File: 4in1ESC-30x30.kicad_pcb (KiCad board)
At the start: 6 copper layers, 41.6 x 42.5 mm, 226 parts, among them J1 SM08B-SRSS-TB, Q1 C22385416, Q10 C22385416, Q11 C22385416, Q12 C22385416, Q13 C22385416, Q14 C22385416, Q15 C22385416, Q16 C22385416, Q17 C22385416, Q18 C22385416, Q19 C22385416, Q2 C22385416, Q20 C22385416, Q21 C22385416, Q22 C22385416, Q23 C22385416, Q24 C22385416, Q3 C22385416, Q4 C22385416, Q5 C22385416, Q6 C22385416, Q7 C22385416, Q8 C22385416, Q9 C22385416, U1 TLV76733DRVR, U10 AT32F421G8U7, U11 NSG2065Q, U12 INA186A3IDCKR, U18 LMR51420YDDCR, U2 AT32F421G8U7, U4 NSG2065Q, U5 XRIM160808SR47MBCD, U6 AT32F421G8U7, U7 NSG2065Q, U8 AT32F421G8U7, U9 NSG2065Q

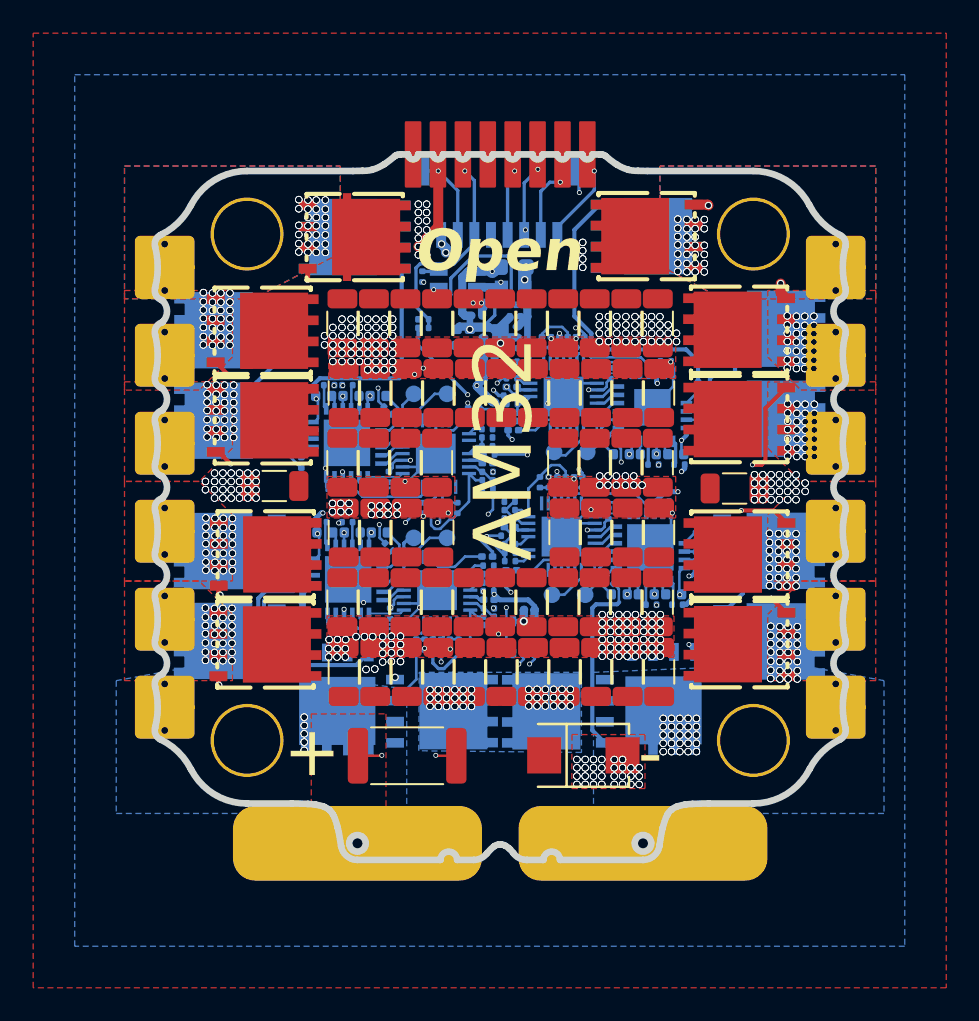
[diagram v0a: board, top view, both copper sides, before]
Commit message: alpha routing
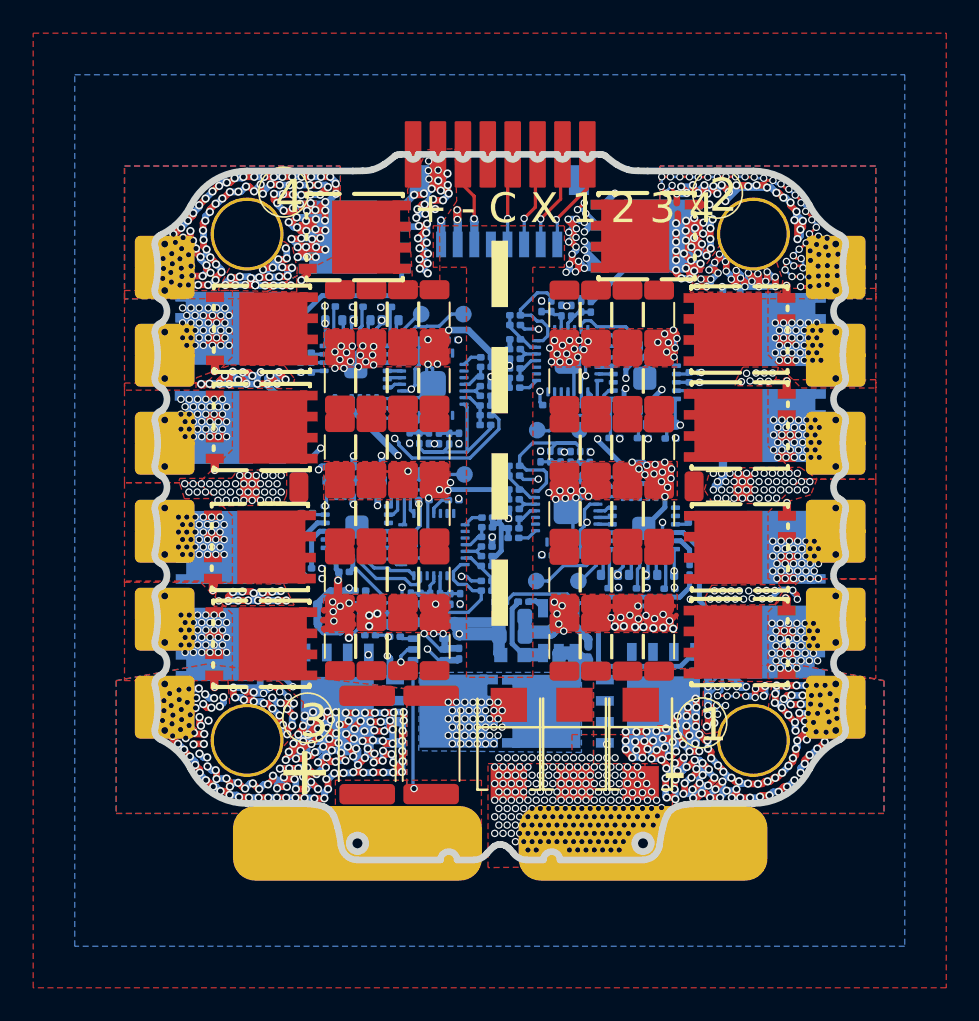
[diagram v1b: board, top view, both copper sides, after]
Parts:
- removed C1, C42: 22uF, Capacitor_SMD:C_0402_1005Metric
- removed C46, C77, C78: 100nF, Capacitor_SMD:C_0201_0603Metric
- removed the C6 at (81.3, 37.5)
- removed the C6 at (83.2, 45.9)
- removed the C6 at (83.2, 37.5)
- removed the C6 at (66.2, 50.1)
- removed the C6 at (70.0, 41.7)
- removed the C6 at (66.2, 41.7)
- removed the C6 at (68.0, 54.3)
- removed the C6 at (73.7, 37.5)
- removed the C6 at (77.6, 58.5)
- removed the C6 at (75.7, 58.5)
- removed the C6 at (68.1, 50.1)
- removed the C6 at (79.5, 41.7)
- removed the C6 at (71.8, 54.3)
- removed the C6 at (85.2, 58.5)
- removed the C6 at (71.8, 37.5)
- removed the C6 at (69.9, 37.5)
- removed the C6 at (71.8, 45.9)
- removed the C6 at (75.7, 41.7)
- removed the C6 at (73.7, 54.3)
- removed the C6 at (77.5, 54.3)
- removed the C6 at (79.5, 58.5)
- removed the C6 at (69.9, 45.9)
- removed the C6 at (81.3, 45.9)
- removed the C6 at (81.3, 54.3)
- removed the C6 at (73.8, 41.7)
- removed the C6 at (83.3, 50.1)
- removed the C6 at (75.6, 54.3)
- removed the C6 at (81.4, 41.7)
- removed the C6 at (75.6, 37.5)
- removed the C6 at (85.1, 54.3)
- removed the C6 at (79.5, 50.1)
- removed the C6 at (71.9, 58.5)
- removed the C6 at (73.8, 58.5)
- removed the C6 at (77.5, 37.5)
- removed the C6 at (79.4, 54.3)
- removed the C6 at (85.1, 37.5)
- removed the C6 at (85.2, 41.7)
- removed the C6 at (85.1, 45.9)
- removed the C6 at (71.9, 50.1)
- removed the C6 at (66.1, 54.3)
- removed the C6 at (83.3, 41.7)
- removed the C6 at (85.2, 50.1)
- removed the C6 at (79.4, 45.9)
- removed the C6 at (81.4, 50.1)
- removed the C6 at (68.1, 41.7)
- removed the C6 at (66.1, 45.9)
- removed the C6 at (68.0, 45.9)
- removed the C6 at (66.1, 37.5)
- removed the C6 at (83.3, 58.5)
- removed the C6 at (70.0, 58.5)
- removed the C6 at (71.9, 41.7)
- removed the C6 at (81.4, 58.5)
- removed the C6 at (79.4, 37.5)
- removed the C6 at (66.2, 58.5)
- removed the C6 at (69.9, 54.3)
- removed the C6 at (68.1, 58.5)
- removed the C6 at (70.0, 50.1)
- removed the C6 at (68.0, 37.5)
- removed the C6 at (77.6, 41.7)
- removed the C6 at (83.2, 54.3)
- removed C73: 100nF, Capacitor_SMD:C_0402_1005Metric
- removed FB1, FB2, FB3, FB4: BLM03PX121SN1D, Inductor_SMD:L_0201_0603Metric
- removed R1, R16, R17, R2, R6, R7, R8, R9: 8R, Capacitor_SMD:C_0201_0603Metric
- removed R118, R3, R4: 10k, Capacitor_SMD:C_0201_0603Metric
- removed R119: 124k, Resistor_SMD:R_0201_0603Metric
- removed R5: 220R, Resistor_SMD:R_0201_0603Metric
- removed U1: TLV76733DRVR, 4in1ESC-30x30:WSON-6_L2.0-W2.0-P0.65-TL-EP
- removed U11: NSG2065Q, 4in1ESC-30x30:QFN-24_L4.0-W4.0-P0.50-TL-EP2.8
- removed U18: LMR51420YDDCR, 4in1ESC-30x30:SOT-23-6_L2.9-W1.6-P0.95-LS2.9-BL
- added C100: 10uF, Capacitor_SMD:C_1206_3216Metric, F.Cu at (69.8, 56.9)
- added C101: 10uF, Capacitor_SMD:C_1206_3216Metric, F.Cu at (71.7, 56.9)
- added C105: 10uF, Capacitor_SMD:C_1206_3216Metric, F.Cu at (79.5, 57.0)
- added C106: 10uF, Capacitor_SMD:C_1206_3216Metric, F.Cu at (81.4, 57.0)
- added C107: 10uF, Capacitor_SMD:C_1206_3216Metric, F.Cu at (83.3, 57.0)
- added C108: 10uF, Capacitor_SMD:C_1206_3216Metric, F.Cu at (85.2, 57.0)
- added C13: 10uF, Capacitor_SMD:C_1206_3216Metric, F.Cu at (85.2, 37.0)
- added C14: 10uF, Capacitor_SMD:C_1206_3216Metric, F.Cu at (83.3, 37.0)
- added C15: 10uF, Capacitor_SMD:C_1206_3216Metric, F.Cu at (81.4, 37.0)
- added C16: 10uF, Capacitor_SMD:C_1206_3216Metric, F.Cu at (79.5, 37.0)
- added C17: 10uF, Capacitor_SMD:C_1206_3216Metric, F.Cu at (66.0, 40.9)
- added C18: 10uF, Capacitor_SMD:C_1206_3216Metric, F.Cu at (67.9, 40.9)
- added C19: 10uF, Capacitor_SMD:C_1206_3216Metric, F.Cu at (69.8, 40.9)
- added C20: 10uF, Capacitor_SMD:C_1206_3216Metric, F.Cu at (71.7, 40.9)
- added C24: 10uF, Capacitor_SMD:C_1206_3216Metric, F.Cu at (79.5, 41.0)
- added C25: 10uF, Capacitor_SMD:C_1206_3216Metric, F.Cu at (81.4, 41.0)
- added C26: 10uF, Capacitor_SMD:C_1206_3216Metric, F.Cu at (83.3, 41.0)
- added C27: 10uF, Capacitor_SMD:C_1206_3216Metric, F.Cu at (85.2, 41.0)
- added C28: 10uF, Capacitor_SMD:C_1206_3216Metric, F.Cu at (71.7, 44.9)
- added C29: 10uF, Capacitor_SMD:C_1206_3216Metric, F.Cu at (69.8, 44.9)
- added C30: 10uF, Capacitor_SMD:C_1206_3216Metric, F.Cu at (67.9, 44.9)
- added C31: 10uF, Capacitor_SMD:C_1206_3216Metric, F.Cu at (66.0, 44.9)
- added C4: 22uF, Capacitor_SMD:C_0402_1005Metric, B.Cu at (65.1, 54.5)
- added C47: 22uF, Capacitor_SMD:C_0603_1608Metric, B.Cu at (76.3, 55.1)
- added C51: 22uF, Capacitor_SMD:C_0402_1005Metric, B.Cu at (65.1, 55.4)
- added C52: 100nF, Capacitor_SMD:C_0201_0603Metric, B.Cu at (76.5, 40.8)
- added C54: 100nF, Capacitor_SMD:C_0201_0603Metric, B.Cu at (76.5, 39.0)
- added C55: 100nF, Capacitor_SMD:C_0201_0603Metric, B.Cu at (80.3, 42.4)
- added C56: 100nF, Capacitor_SMD:C_0402_WIDE, B.Cu at (82.3, 43.6)
- added C58: 100nF, Capacitor_SMD:C_0201_0603Metric, B.Cu at (85.1, 38.1)
- added C6: 10uF, Capacitor_SMD:C_1206_3216Metric, F.Cu at (79.5, 45.0)
- added C6: 10uF, Capacitor_SMD:C_1206_3216Metric, F.Cu at (71.7, 36.9)
- added C6: 10uF, Capacitor_SMD:C_1206_3216Metric, F.Cu at (71.7, 52.9)
- added C60: 100nF, Capacitor_SMD:C_0201_0603Metric, B.Cu at (74.8, 51.5)
- added C61: 100nF, Capacitor_SMD:C_0201_0603Metric, B.Cu at (71.0, 48.1)
- added C62: 100nF, Capacitor_SMD:C_0402_WIDE, B.Cu at (69.1, 46.9)
- added C67: 100nF, Capacitor_SMD:C_0402_WIDE, B.Cu at (69.0, 37.3)
- added C68: 100nF, Capacitor_SMD:C_0201_0603Metric, B.Cu at (66.2, 42.8)
- added C7: 10uF, Capacitor_SMD:C_1206_3216Metric, F.Cu at (69.8, 36.9)
- added C74: 100nF, Capacitor_SMD:C_0201_0603Metric, B.Cu at (80.9, 57.3)
- added C75: 100nF, Capacitor_SMD:C_0201_0603Metric, B.Cu at (77.0, 54.2)
- added C76: 100nF, Capacitor_SMD:C_0201_0603Metric, B.Cu at (69.3, 55.3)
- added C8: 10uF, Capacitor_SMD:C_1206_3216Metric, F.Cu at (67.9, 36.9)
- added C81: 100nF, Capacitor_SMD:C_0201_0603Metric, B.Cu at (67.2, 53.6)
- added C82: 10uF, Capacitor_SMD:C_1206_3216Metric, F.Cu at (83.3, 49.0)
- added C84: 10uF, Capacitor_SMD:C_1206_3216Metric, F.Cu at (85.2, 52.9)
- added C85: 10uF, Capacitor_SMD:C_1206_3216Metric, F.Cu at (83.3, 52.9)
- added C86: 22uF, Capacitor_SMD:C_0603_1608Metric, B.Cu at (76.3, 56.3)
- added C87: 10uF, Capacitor_SMD:C_1206_3216Metric, F.Cu at (81.4, 52.9)
- added C9: 10uF, Capacitor_SMD:C_1206_3216Metric, F.Cu at (66.0, 36.9)
- added C95: 10uF, Capacitor_SMD:C_1206_3216Metric, F.Cu at (69.8, 52.9)
- added C96: 10uF, Capacitor_SMD:C_1206_3216Metric, F.Cu at (67.9, 52.9)
- added C97: 10uF, Capacitor_SMD:C_1206_3216Metric, F.Cu at (66.0, 52.9)
- added C98: 10uF, Capacitor_SMD:C_1206_3216Metric, F.Cu at (66.0, 56.9)
- added C99: 10uF, Capacitor_SMD:C_1206_3216Metric, F.Cu at (67.9, 56.9)
- added D2: SMBJ24A, 4in1ESC-30x30:SMB_L4.5-W3.7-LS5.4-RD, F.Cu at (80.1, 62.8)
- added D3: SMBJ24A, 4in1ESC-30x30:SMB_L4.5-W3.7-LS5.4-RD, F.Cu at (76.2, 62.8)
- added R120: 115k, Resistor_SMD:R_0201_0603Metric, B.Cu at (75.6, 54.3)
- added R121: 10k, 4in1ESC:R_0201_0603Metric, B.Cu at (80.9, 54.6)
- added R74: 15R, Resistor_SMD:R_0201_0603Metric, B.Cu at (64.6, 52.8)
- added R75: 15R, Resistor_SMD:R_0201_0603Metric, B.Cu at (63.9, 39.8)
- added R76: 15R, Resistor_SMD:R_0201_0603Metric, B.Cu at (82.5, 53.4)
- added R77: 15R, Resistor_SMD:R_0201_0603Metric, B.Cu at (82.5, 44.4)
- added R78: 15R, Resistor_SMD:R_0201_0603Metric, B.Cu at (68.8, 46.1)
- added R79: 15R, Resistor_SMD:R_0201_0603Metric, B.Cu at (68.8, 36.5)
- added R80: 15R, Resistor_SMD:R_0201_0603Metric, B.Cu at (87.0, 52.3)
- added R81: 15R, Resistor_SMD:R_0201_0603Metric, B.Cu at (87.3, 41.6)
- added R82: 15R, Resistor_SMD:R_0201_0603Metric, B.Cu at (64.0, 48.9)
- added R83: 15R, Resistor_SMD:R_0201_0603Metric, B.Cu at (63.9, 39.2)
- added R84: 10R, Resistor_SMD:R_0201_0603Metric, B.Cu at (76.5, 48.7)
- added R85: 10R, Resistor_SMD:R_0201_0603Metric, B.Cu at (76.5, 39.6)
- added R86: 10R, Resistor_SMD:R_0201_0603Metric, B.Cu at (74.8, 50.9)
- added R87: 220R, Resistor_SMD:R_0201_0603Metric, B.Cu at (72.8, 38.5)
- added R88: 10R, Resistor_SMD:R_0201_0603Metric, B.Cu at (74.8, 41.3)
- added Rsense2: 0.2mR, Resistor_SMD:R_2512_6332Metric, F.Cu at (71.5, 62.9)
- added U13: LMR54406DBVR, 4in1ESC:SOT-23-6_L2.9-W1.6-P0.95-LS2.8-BR, B.Cu at (79.2, 56.0)
- added U14: FTC160808S4R7MBCA, 4in1ESC:IND-SMD_L1.6-W0.8_FTC160865SR47MBCA, B.Cu at (76.4, 57.5)
- added U15: TLV76733DRVR, 4in1ESC:WSON-6_L2.0-W2.0-P0.65-TL-EP, B.Cu at (67.5, 55.0)
- C32, C33, C34, C35, C36, C37, C38, C39, C53: footprint Capacitor_SMD:C_0402_1005Metric -> Capacitor_SMD:C_0402_WIDE
- C43: value 22uF -> 10uF; footprint Capacitor_SMD:C_0603_1608Metric -> Capacitor_SMD:C_1206_3216Metric; moved to F.Cu
- C44, C45, C69, C70, C71, C72, C79, C80, C88: value 100nF -> 10uF; footprint Capacitor_SMD:C_0201_0603Metric -> Capacitor_SMD:C_1206_3216Metric; moved to F.Cu
- C59: footprint Capacitor_SMD:C_0402_1005Metric -> Capacitor_SMD:C_0201_0603Metric
- C83: value 100nF -> 10uF; footprint Capacitor_SMD:C_0402_1005Metric -> Capacitor_SMD:C_1206_3216Metric; moved to F.Cu
- D1: value SMBJ26A_C908802 -> SMBJ24A
- R18, R19, R40, R58: footprint Capacitor_SMD:C_0201_0603Metric -> Resistor_SMD:R_0201_0603Metric
- R21, R22: value 8R -> 10k; footprint Capacitor_SMD:C_0201_0603Metric -> Resistor_SMD:R_0201_0603Metric
- R23, R24, R37, R38, R42, R43, R44, R45, R55, R56, R60, R61, R62, R63: value 8R -> 15R; footprint Capacitor_SMD:C_0201_0603Metric -> Resistor_SMD:R_0201_0603Metric
- R39, R57: value 10k -> 220R; footprint Capacitor_SMD:C_0201_0603Metric -> Resistor_SMD:R_0201_0603Metric
- R41, R59: value 220R -> 10k
- U10, U6, U8: value AT32F421G8U7 -> NSG2065Q; footprint 4in1ESC-30x30:QFN-28_L4.0-W4.0-P0.40-TL-EP2.4 -> 4in1ESC:QFN-24_L4.0-W4.0-P0.50-TL-EP2.8
- U2: footprint 4in1ESC-30x30:QFN-28_L4.0-W4.0-P0.40-TL-EP2.4 -> 4in1ESC:QFN-28_L4.0-W4.0-P0.40-TL-EP2.4
- U4: footprint 4in1ESC-30x30:QFN-24_L4.0-W4.0-P0.50-TL-EP2.8 -> 4in1ESC:QFN-24_L4.0-W4.0-P0.50-TL-EP2.8
- U5: value XRIM160808SR47MBCD -> AT32F421G8U7; footprint 4in1ESC-30x30:IND-SMD_L1.6-W0.8_FTC160865SR47MBCA -> 4in1ESC:QFN-28_L4.0-W4.0-P0.40-TL-EP2.4
- U7, U9: value NSG2065Q -> AT32F421G8U7; footprint 4in1ESC-30x30:QFN-24_L4.0-W4.0-P0.50-TL-EP2.8 -> 4in1ESC:QFN-28_L4.0-W4.0-P0.40-TL-EP2.4
- moved R63 24.2 mm to (87.3, 41.0), turned to 0 degrees
- moved R42 24.1 mm to (87.3, 49.5), turned to 0 degrees
- moved R62 24.0 mm to (87.6, 52.3)
- moved C63 23.2 mm to (66.2, 52.4), turned to 180 degrees
- moved R44 22.7 mm to (64.6, 52.2)
- moved R61 21.1 mm to (67.0, 36.5), turned to 180 degrees
- moved R60 20.6 mm to (67.1, 46.1), turned to 180 degrees
- moved C94 19.3 mm to (67.8, 56.3)
- moved R56 19.2 mm to (84.2, 44.4)
- moved R55 18.7 mm to (84.2, 53.4), turned to 0 degrees
- moved R73 18.7 mm to (69.3, 56.4), turned to 0 degrees
- moved C83 18.4 mm to (85.2, 49.0), turned to 90 degrees
- moved R38 16.6 mm to (65.4, 36.5), turned to 180 degrees
- moved U7 15.6 mm to (71.6, 50.8), turned to 180 degrees
- moved C88 14.9 mm to (79.5, 52.9), turned to -90 degrees
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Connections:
- C33 pad 2: Net-(U7-VB2) -> Net-(U6-VB2)
- C34 pad 2: Net-(U9-VB2) -> Net-(U8-VB2)
- C35 pad 2: Net-(U11-VB2) -> Net-(U10-VB2)
- C37 pad 2: Net-(U7-VB3) -> Net-(U6-VB3)
- C38 pad 2: Net-(U9-VB3) -> Net-(U8-VB3)
- C39 pad 2: Net-(U11-VB3) -> Net-(U10-VB3)
- C43 pad 1: +8V -> +BATT
- C44 pad 1: +3V3 -> +BATT
- C45 pad 1: +3V3 -> +BATT
- C48 pad 1: +3V3 -> /ESC1/vdda
- C57 pad 1: +8V -> +10V
- C59 pad 1: /ESC2/MotorA -> Net-(U7-NRST)
- C59 pad 2: Net-(U7-VB1) -> GND
- C63 pad 1: +8V -> +10V
- C64 pad 1: +3V3 -> Net-(U9-NRST)
- C65 pad 1: +3V3 -> /ESC4/vdda
- C66 pad 1: Net-(U8-NRST) -> +3V3
- C70 pad 1: +8V -> +BATT
- C71 pad 1: +3V3 -> +BATT
- C72 pad 1: Net-(U18-SW) -> +BATT
- C72 pad 2: Net-(U18-CB) -> GND
- C79 pad 1: +3V3 -> +BATT
- C80 pad 1: Net-(U10-NRST) -> +BATT
- C83 pad 1: /ESC4/MotorA -> +BATT
- C83 pad 2: Net-(U11-VB1) -> GND
- C88 pad 1: +8V -> +BATT
- R21 pad 1: /ESC3/GHB -> Net-(U5-NRST)
- R21 pad 2: Net-(Q9-G) -> +3V3
- R22 pad 1: /ESC4/GHB -> Net-(U5-BOOT0)
- R22 pad 2: Net-(Q10-G) -> GND
- R23 pad 1: /ESC1/GLB -> /ESC1/GHC
- R23 pad 2: Net-(Q11-G) -> Net-(Q16-G)
- R24 pad 1: /ESC2/GLB -> /ESC2/GHC
- R24 pad 2: Net-(Q12-G) -> Net-(Q17-G)
- R37 pad 1: /ESC3/GHA -> /ESC3/GHC
- R37 pad 2: Net-(Q13-G) -> Net-(Q18-G)
- R38 pad 1: /ESC3/GLB -> /ESC4/GHC
- R38 pad 2: Net-(Q14-G) -> Net-(Q20-G)
- R39 pad 1: Net-(U8-NRST) -> /M2
- R39 pad 2: +3V3 -> Net-(U5-PB4)
- R40 pad 1: Net-(U8-BOOT0) -> Net-(U7-NRST)
- R40 pad 2: GND -> +3V3
- R41 pad 1: /M3 -> Net-(U7-BOOT0)
- R41 pad 2: Net-(U8-PB4) -> GND
- R42 pad 1: /ESC4/GLB -> /ESC1/GLC
- R42 pad 2: Net-(Q15-G) -> Net-(Q21-G)
- R43 pad 1: /ESC1/GHC -> /ESC2/GLC
- R43 pad 2: Net-(Q16-G) -> Net-(Q22-G)
- R44 pad 1: /ESC2/GHC -> /ESC3/GLC
- R44 pad 2: Net-(Q17-G) -> Net-(Q23-G)
- R45 pad 1: /ESC3/GHC -> /ESC4/GLC
- R45 pad 2: Net-(Q18-G) -> Net-(Q24-G)
- R55 pad 1: /ESC4/GHA -> /ESC1/GHB
- R55 pad 2: Net-(Q19-G) -> Net-(Q6-G)
- R56 pad 1: /ESC4/GHC -> /ESC2/GHB
- R56 pad 2: Net-(Q20-G) -> Net-(Q8-G)
- R57 pad 1: Net-(U10-NRST) -> /M3
- R57 pad 2: +3V3 -> Net-(U7-PB4)
- R58 pad 1: Net-(U10-BOOT0) -> Net-(U9-NRST)
- R58 pad 2: GND -> +3V3
- R59 pad 1: /M4 -> Net-(U9-BOOT0)
- R59 pad 2: Net-(U10-PB4) -> GND
- R60 pad 1: /ESC1/GLC -> /ESC3/GHB
- R60 pad 2: Net-(Q21-G) -> Net-(Q9-G)
- R61 pad 1: /ESC2/GLC -> /ESC4/GHB
- R61 pad 2: Net-(Q22-G) -> Net-(Q10-G)
- R62 pad 1: /ESC3/GLC -> /ESC1/GLB
- R62 pad 2: Net-(Q23-G) -> Net-(Q11-G)
- R63 pad 1: /ESC4/GLC -> /ESC2/GLB
- R63 pad 2: Net-(Q24-G) -> Net-(Q12-G)
- TP2 pad 1: Net-(U6-PA13) -> Net-(U5-PA13)
- TP3 pad 1: Net-(U6-PA14) -> Net-(U7-PA13)
- TP5 pad 1: Net-(U8-PA13) -> Net-(U5-PA14)
- TP6 pad 1: Net-(U8-PA14) -> Net-(U7-PA14)
- TP7 pad 1: Net-(U10-PA13) -> Net-(U9-PA13)
- TP8 pad 1: Net-(U10-PA14) -> Net-(U9-PA14)
- U10 pad 1: Net-(U10-BOOT0) -> /ESC4/AL
- U10 pad 10: /ESC4/FBB -> /ESC4/GLB
- U10 pad 11: /ESC4/FBC -> /ESC4/GLA
- U10 pad 12: unconnected-(U10-PA6-Pad12) -> /ESC4/MotorC
- U10 pad 13: /ESC4/CL -> /ESC4/GHC
- U10 pad 14: /ESC4/BL -> Net-(U10-VB3)
- U10 pad 15: /ESC4/AL -> /ESC4/MotorB
- U10 pad 16: GND -> /ESC4/GHB
- U10 pad 17: +3V3 -> Net-(U10-VB2)
- U10 pad 18: /ESC4/CH -> /ESC4/MotorA
- U10 pad 19: /ESC4/BH -> /ESC4/GHA
- U10 pad 2: unconnected-(U10-PF0/OSC_IN-Pad2) -> /ESC4/BL
- U10 pad 20: /ESC4/AH -> Net-(U10-VB1)
- U10 pad 21: Net-(U10-PA13) -> unconnected-(U10-NC-Pad21)
- U10 pad 22: Net-(U10-PA14) -> /ESC4/AH
- U10 pad 23: unconnected-(U10-PA15-Pad23) -> /ESC4/BH
- U10 pad 24: unconnected-(U10-PB3-Pad24) -> /ESC4/CH
- U10 pad 25: Net-(U10-PB4) -> GND
- U10 pad 4: Net-(U10-NRST) -> +10V
- U10 pad 6: /ESC4/FBA -> GND
- U10 pad 9: unconnected-(U10-PA3-Pad9) -> /ESC4/GLC
- U2 pad 5: Net-(U2-VDDA) -> /ESC1/vdda
- U4 pad 4: +8V -> +10V
- U5 pad 1: Net-(U18-SW) -> Net-(U5-BOOT0)
- U5 pad 2: +8V -> unconnected-(U5-PF0/OSC_IN-Pad2)
- U6 pad 1: Net-(U6-BOOT0) -> /ESC2/AL
- U6 pad 10: /ESC2/FBB -> /ESC2/GLB
- U6 pad 11: /ESC2/FBC -> /ESC2/GLA
- U6 pad 12: unconnected-(U6-PA6-Pad12) -> /ESC2/MotorC
- U6 pad 13: /ESC2/CL -> /ESC2/GHC
- U6 pad 14: /ESC2/BL -> Net-(U6-VB3)
- U6 pad 15: /ESC2/AL -> /ESC2/MotorB
- U6 pad 16: GND -> /ESC2/GHB
- U6 pad 17: +3V3 -> Net-(U6-VB2)
- U6 pad 18: /ESC2/CH -> /ESC2/MotorA
- U6 pad 19: /ESC2/BH -> /ESC2/GHA
- U6 pad 2: unconnected-(U6-PF0/OSC_IN-Pad2) -> /ESC2/BL
- U6 pad 20: /ESC2/AH -> Net-(U6-VB1)
- U6 pad 21: Net-(U6-PA13) -> unconnected-(U6-NC-Pad21)
- U6 pad 22: Net-(U6-PA14) -> /ESC2/AH
- U6 pad 23: unconnected-(U6-PA15-Pad23) -> /ESC2/BH
- U6 pad 24: unconnected-(U6-PB3-Pad24) -> /ESC2/CH
- U6 pad 25: Net-(U6-PB4) -> GND
- U6 pad 4: Net-(U6-NRST) -> +10V
- U6 pad 6: /ESC2/FBA -> GND
- U6 pad 9: unconnected-(U6-PA3-Pad9) -> /ESC2/GLC
- U7 pad 1: /ESC2/AL -> Net-(U7-BOOT0)
- U7 pad 10: /ESC2/GLB -> /ESC3/FBB
- U7 pad 11: /ESC2/GLA -> /ESC3/FBC
- U7 pad 12: /ESC2/MotorC -> unconnected-(U7-PA6-Pad12)
- U7 pad 13: /ESC2/GHC -> /ESC3/CL
- U7 pad 14: Net-(U7-VB3) -> /ESC3/BL
- U7 pad 15: /ESC2/MotorB -> /ESC3/AL
- U7 pad 16: /ESC2/GHB -> GND
- U7 pad 17: Net-(U7-VB2) -> +3V3
- U7 pad 18: /ESC2/MotorA -> /ESC3/CH
- U7 pad 19: /ESC2/GHA -> /ESC3/BH
- U7 pad 2: /ESC2/BL -> unconnected-(U7-PF0/OSC_IN-Pad2)
- U7 pad 20: Net-(U7-VB1) -> /ESC3/AH
- U7 pad 21: unconnected-(U7-NC-Pad21) -> Net-(U7-PA13)
- U7 pad 22: /ESC2/AH -> Net-(U7-PA14)
- U7 pad 25: GND -> Net-(U7-PB4)
- U7 pad 3: /ESC2/CL -> unconnected-(U7-PF1/OSC_OUT-Pad3)
- U7 pad 4: +8V -> Net-(U7-NRST)
- U7 pad 5: unconnected-(U7-NC-Pad5) -> /ESC3/vdda
- U7 pad 6: GND -> /ESC3/FBA
- U7 pad 9: /ESC2/GLC -> unconnected-(U7-PA3-Pad9)
- U8 pad 1: Net-(U8-BOOT0) -> /ESC3/AL
- U8 pad 10: /ESC3/FBB -> /ESC3/GLB
- U8 pad 11: /ESC3/FBC -> /ESC3/GLA
- U8 pad 12: unconnected-(U8-PA6-Pad12) -> /ESC3/MotorC
- U8 pad 13: /ESC3/CL -> /ESC3/GHC
- U8 pad 14: /ESC3/BL -> Net-(U8-VB3)
- U8 pad 15: /ESC3/AL -> /ESC3/MotorB
- U8 pad 16: GND -> /ESC3/GHB
- U8 pad 17: +3V3 -> Net-(U8-VB2)
- U8 pad 18: /ESC3/CH -> /ESC3/MotorA
- U8 pad 19: /ESC3/BH -> /ESC3/GHA
- U8 pad 2: unconnected-(U8-PF0/OSC_IN-Pad2) -> /ESC3/BL
- U8 pad 20: /ESC3/AH -> Net-(U8-VB1)
- U8 pad 21: Net-(U8-PA13) -> unconnected-(U8-NC-Pad21)
- U8 pad 22: Net-(U8-PA14) -> /ESC3/AH
- U8 pad 23: unconnected-(U8-PA15-Pad23) -> /ESC3/BH
- U8 pad 24: unconnected-(U8-PB3-Pad24) -> /ESC3/CH
- U8 pad 25: Net-(U8-PB4) -> GND
- U8 pad 4: Net-(U8-NRST) -> +10V
- U8 pad 5: Net-(U8-VDDA) -> unconnected-(U8-NC-Pad5)
- U8 pad 6: /ESC3/FBA -> GND
- U8 pad 7: /ESC3/FBCOMMON -> unconnected-(U8-NC-Pad7)
- U8 pad 9: unconnected-(U8-PA3-Pad9) -> /ESC3/GLC
- U9 pad 1: /ESC3/AL -> Net-(U9-BOOT0)
- U9 pad 10: /ESC3/GLB -> /ESC4/FBB
- U9 pad 11: /ESC3/GLA -> /ESC4/FBC
- U9 pad 12: /ESC3/MotorC -> unconnected-(U9-PA6-Pad12)
- U9 pad 13: /ESC3/GHC -> /ESC4/CL
- U9 pad 14: Net-(U9-VB3) -> /ESC4/BL
- U9 pad 15: /ESC3/MotorB -> /ESC4/AL
- U9 pad 16: /ESC3/GHB -> GND
- U9 pad 17: Net-(U9-VB2) -> +3V3
- U9 pad 18: /ESC3/MotorA -> /ESC4/CH
- U9 pad 19: /ESC3/GHA -> /ESC4/BH
- U9 pad 2: /ESC3/BL -> unconnected-(U9-PF0/OSC_IN-Pad2)
- U9 pad 20: Net-(U9-VB1) -> /ESC4/AH
- U9 pad 21: unconnected-(U9-NC-Pad21) -> Net-(U9-PA13)
- U9 pad 22: /ESC3/AH -> Net-(U9-PA14)
- U9 pad 25: GND -> Net-(U9-PB4)
- U9 pad 3: /ESC3/CL -> unconnected-(U9-PF1/OSC_OUT-Pad3)
- U9 pad 4: +8V -> Net-(U9-NRST)
- U9 pad 5: unconnected-(U9-NC-Pad5) -> /ESC4/vdda
- U9 pad 6: GND -> /ESC4/FBA
- U9 pad 9: /ESC3/GLC -> unconnected-(U9-PA3-Pad9)
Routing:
- net GND: track 77.9 -> 295.7 mm, vias 610 -> 592
- net /ESC3/MotorC: track 21.8 -> 129.3 mm, vias 11 -> 166
- net /ESC4/MotorA: track 29.9 -> 102.7 mm, vias 56 -> 110
- net /ESC2/MotorC: track 24.2 -> 95.8 mm, vias 56 -> 108
- net +10V: track 0.00 -> 64.8 mm, vias 0 -> 4
- net /ESC1/MotorA: track 46.3 -> 110.2 mm, vias 52 -> 136
- net +8V: track 59.9 -> 0.00 mm, vias 6 -> 0
- net +3V3: track 60.6 -> 88.0 mm, vias 12 -> 10
- net Net-(U12-OUT): track 22.6 -> 0.82 mm, vias 2 -> 0
- net /CURR: track 12.7 -> 33.6 mm, vias 1 -> 2
- net /ESC2/MotorA: track 34.0 -> 21.4 mm, vias 58 -> 38
- net /ESC1/MotorC: track 26.8 -> 16.0 mm, vias 58 -> 39
- net Net-(Q2-G): track 5.88 -> 16.4 mm, vias 2 -> 0
- net Net-(U18-FB): track 9.75 -> 0.00 mm
- net /ESC4/MotorB: track 31.1 -> 22.7 mm, vias 58 -> 38
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- added copper zone on F.Cu, net /ESC1/MotorA
- added copper zone on In2.Cu, net /ESC1/MotorA
- added copper zone on In3.Cu, net /ESC1/MotorA
- added copper zone on In2.Cu, net /ESC2/MotorC
- added copper zone on In3.Cu, net /ESC2/MotorC
- added copper zone on F.Cu, net /ESC3/MotorC
- added copper zone on In2.Cu, net /ESC3/MotorC
- added copper zone on In3.Cu, net /ESC3/MotorC
- added copper zone on In2.Cu, net /ESC4/MotorA
- added copper zone on In3.Cu, net /ESC4/MotorA
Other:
- board text added: "+ - C X 1 2 3 4"
- board text added: "1"
- board text added: "2"
- board text added: "3"
- board text added: "4"
- board text added: "4 3 2 1 X C - +"
- board text removed: "3-6S INPUT"
- board text removed: "4 3 2 1 T C - +"
- board text removed: "AM32"
